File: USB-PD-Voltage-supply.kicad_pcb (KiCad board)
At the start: 4 copper layers, 73.6 x 70.6 mm, 231 parts, among them J1 DC-005-5A-2.5-SMT, J2 Conn_01x07_Pin, J3 Conn_01x04_Pin, J4 TYPE-C-31-M-31, J5 Conn_01x11_Pin, J6 Conn_01x11_Pin, J7 Conn_01x11_Pin, Q1 STL6P3LLH6, Q2 STL6P3LLH6, SW1 TS-1088-AR02016, SW2 TS-1088-AR02016, U1 AP1117-33, U10 TPS55289RYQR, U11 TPS55289RYQR, U12 LMR16030PDDAR, U13 LMR16030PDDAR, U2 ESP32-C3, U3 STUSB4500QTR, U4 PCA9555PW, U5 W25Q128JVS, U6 INA180A2, U7 INA180A2, U8 INA180A2, U9 INA180A2, Y1 X322540MPB4SI

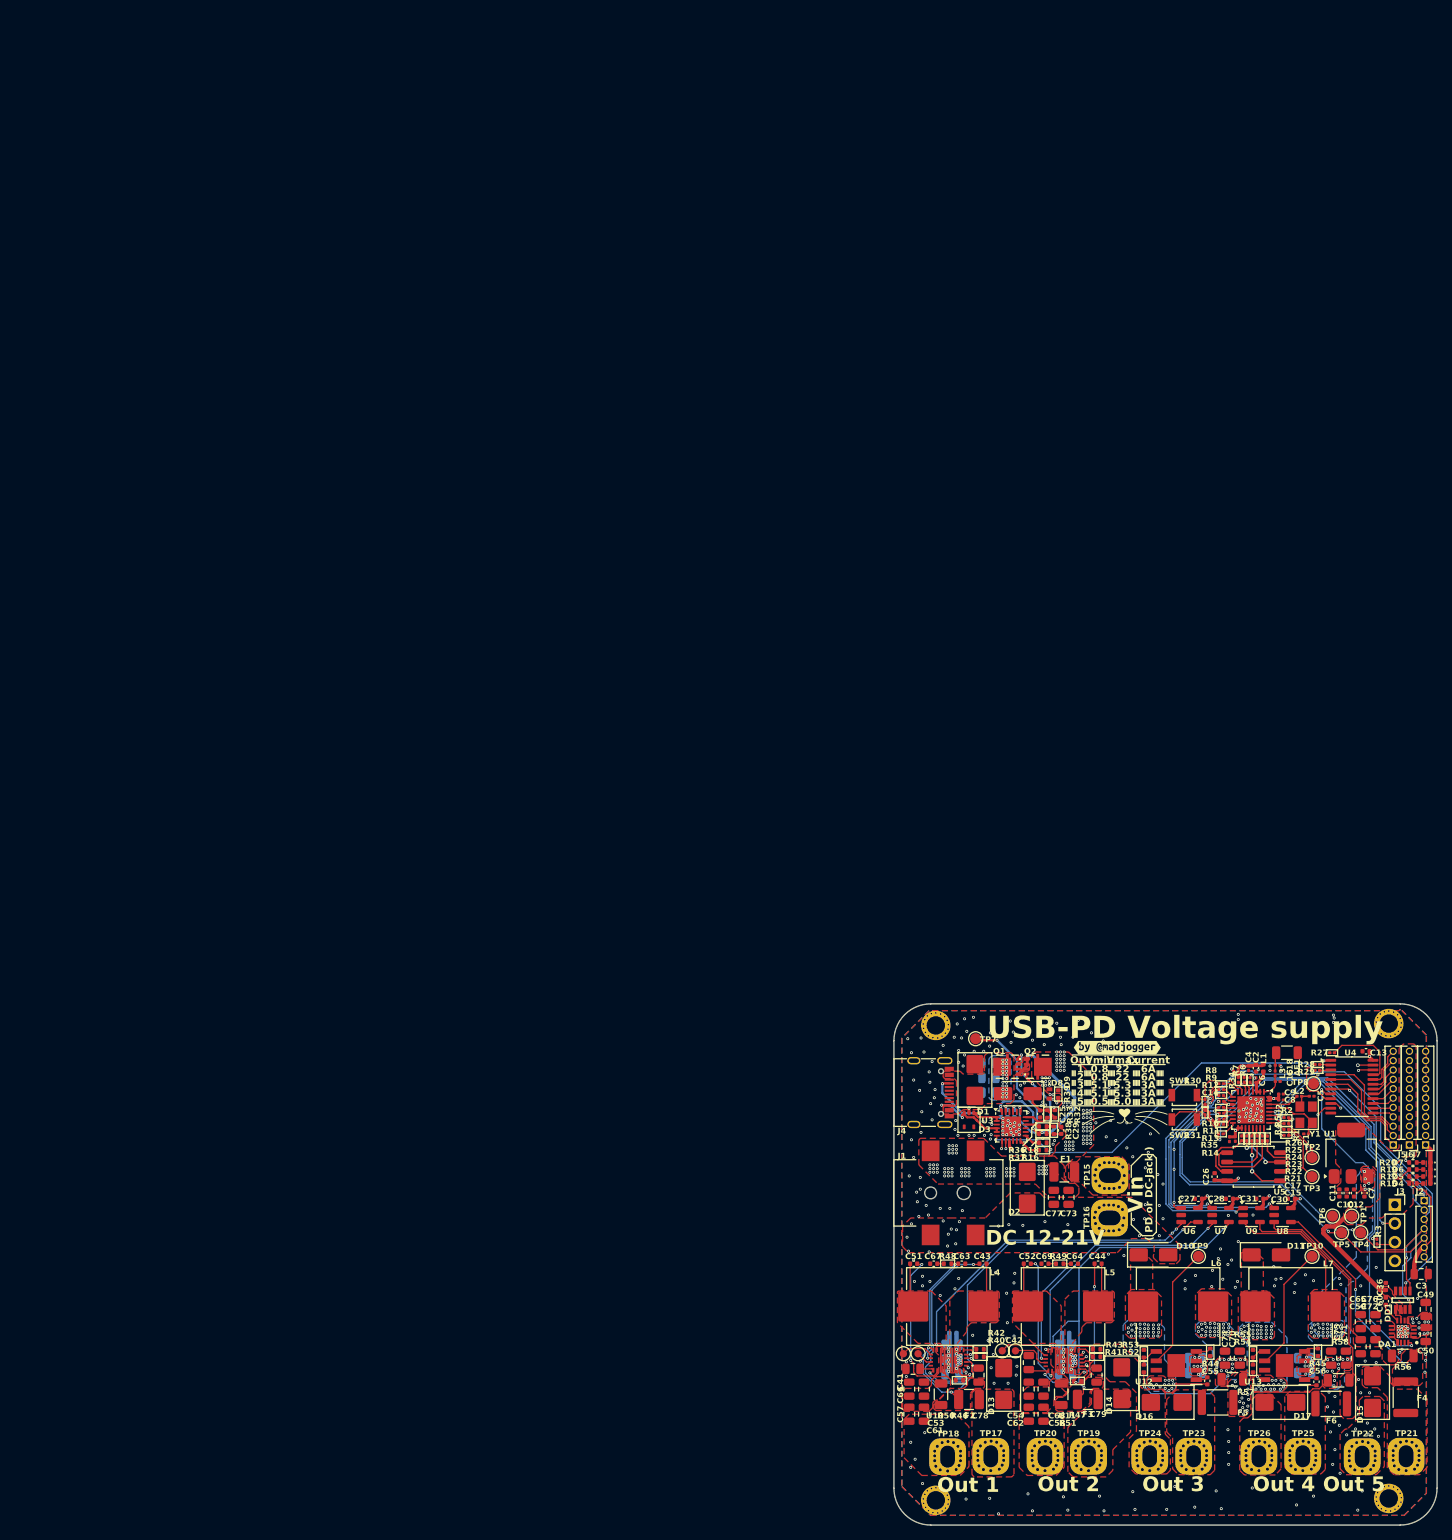
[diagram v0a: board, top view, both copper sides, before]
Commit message: added simulation data for CST + design update ( no important changes )
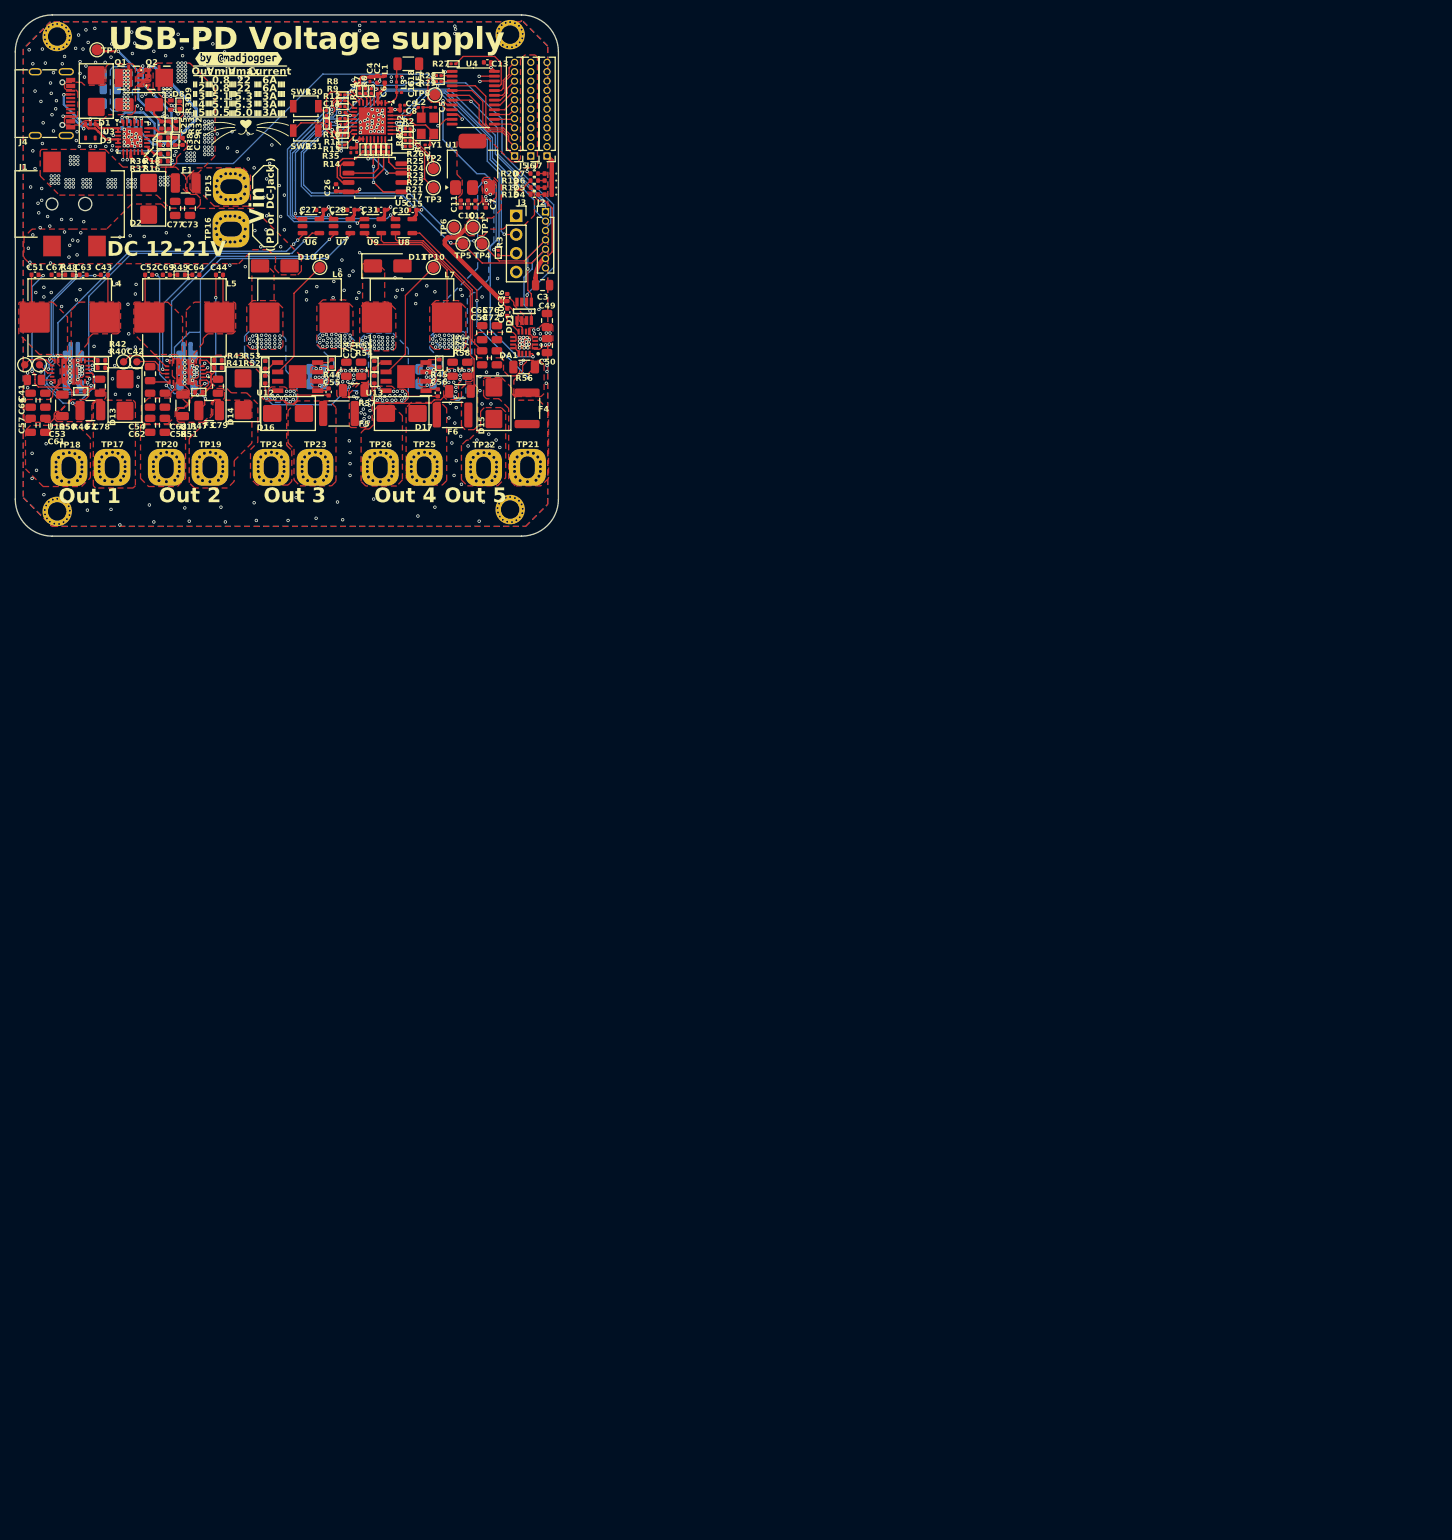
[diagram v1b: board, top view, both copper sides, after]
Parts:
- moved ? 179.3 mm to (6.10, -68.5)
- moved ? 179.3 mm to (6.10, -4.18)
- moved AE1 179.3 mm to (53.7, -64.8)
- moved C1 179.3 mm to (56.3, -53.9)
- moved C10 179.3 mm to (61.8, -45.8)
- moved C11 179.3 mm to (60.8, -45.8)
- moved C12 179.3 mm to (62.8, -45.8)
- moved C13 179.3 mm to (64.4, -65.0)
- moved C16 179.3 mm to (52.5, -61.0)
- moved C17 179.3 mm to (46.7, -53.2)
- moved C19 179.3 mm to (15.8, -56.6)
- moved C22 179.3 mm to (13.3, -59.5)
- moved C23 179.3 mm to (13.3, -63.5)
- moved C24 179.3 mm to (13.3, -61.5)
- moved C27 179.3 mm to (41.7, -45.0)
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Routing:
- net Net-(U3-ALERT): track 23.0 -> 23.5 mm
- net CURR_SENSE_1: vias 4 -> 2
